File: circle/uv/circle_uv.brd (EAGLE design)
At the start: 27.9 x 39.4 mm, 7 parts

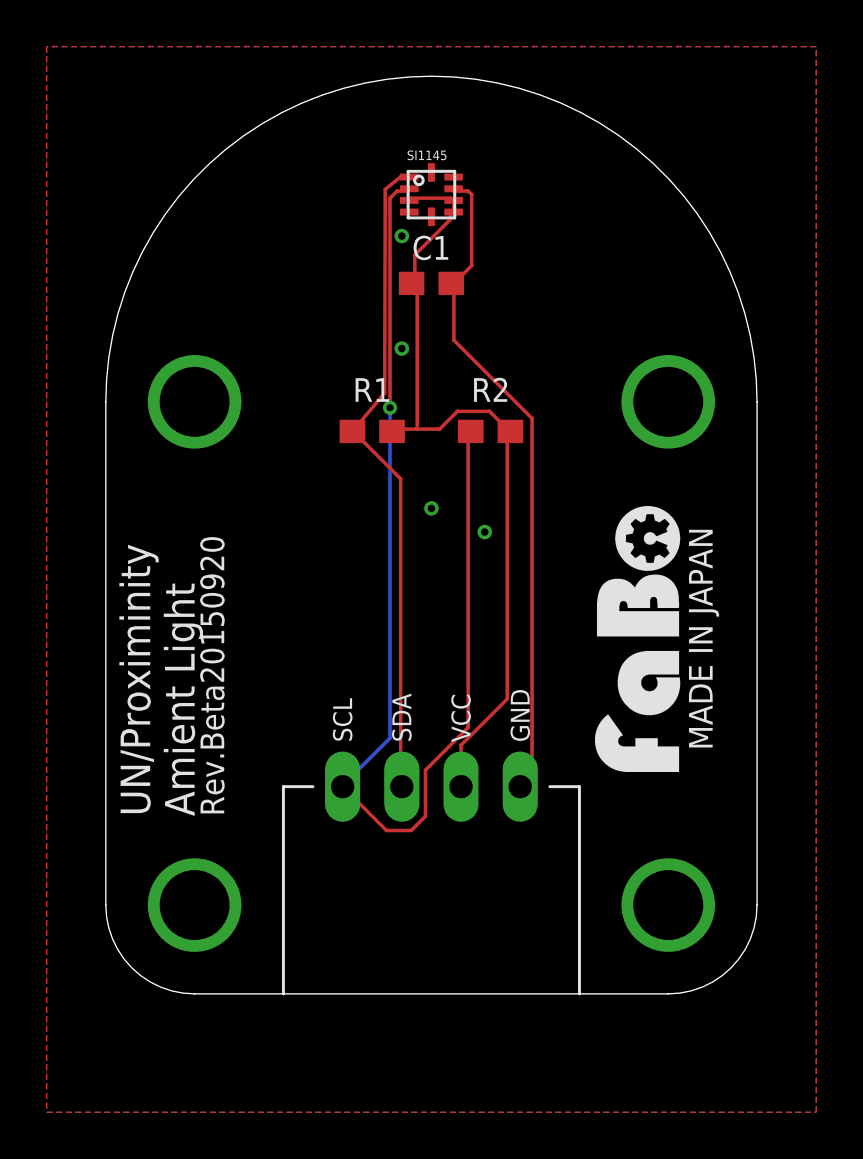
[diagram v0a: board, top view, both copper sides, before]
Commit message: Update circle
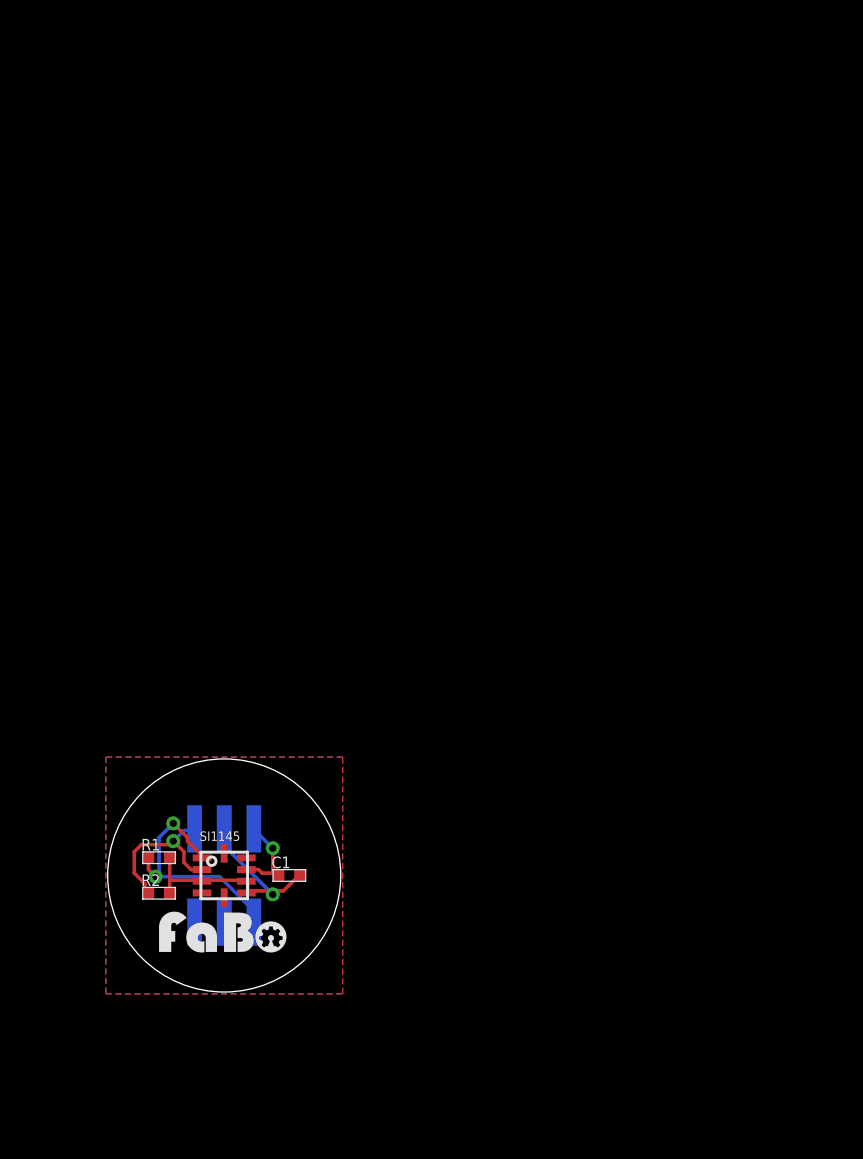
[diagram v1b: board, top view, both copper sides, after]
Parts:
- removed J1: (no value), GClue:BRICK_I2C
- removed U$4: (no value), GClue:LOGO_OSHW_T_M_BOTTOM
- added U$2: FABO-NANO, FaBo-Template:FABO-NANO
- C1: value 0.1uF -> 0.1uf; device GClue:EIA0603 -> FaBo-Capacitor:0402
- R1, R2: value 4.7k -> 4.7K; device GClue:EIA0603 -> FaBo-Resistors:0402
- U$3: device FaBo:LOGO_FABO_M -> FaBo-etc:LOGO_FABO_S
- moved SI1145 30.5 mm to (5.08, 5.08)
- moved C1 26.1 mm to (7.87, 5.08)
- moved R2 24.4 mm to (2.29, 4.32)
- moved U$3 23.7 mm to (5.08, 1.78), turned to 0 degrees
- moved R1 20.4 mm to (2.29, 5.84)
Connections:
- net 3V3: now also C1.P$2, R1.P$2, R2.P$2, U$2.VCC; no longer C1.1, J1.VCC, R1.2, R2.2
- net GND: now also C1.P$1, U$2.GND; no longer C1.2, J1.GND
- net SCL: now also R2.P$1, U$2.0; no longer J1.SCL, R2.1
- net SDA: now also R1.P$1, U$2.1; no longer J1.SDA, R1.1
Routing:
- net SCL: track 49.0 -> 7.12 mm
- net GND: track 28.3 -> 3.72 mm, vias 4 -> 1
- net 3V3: track 34.9 -> 11.7 mm, vias 0 -> 1
- net SDA: track 28.2 -> 10.8 mm, vias 0 -> 2
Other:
- board size 27.9 x 39.4 mm -> 10 x 10 mm
- board text removed: "MADE IN JAPAN"
- board text removed: "Rev.Beta20150920"
- board text removed: "UN/Proximinity Amient Light"
